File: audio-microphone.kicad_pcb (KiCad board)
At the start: 2 copper layers, 20 x 20 mm, 9 parts, among them J1 JST_SH_1x4_BM04B-SRSS-TB-LF-SN

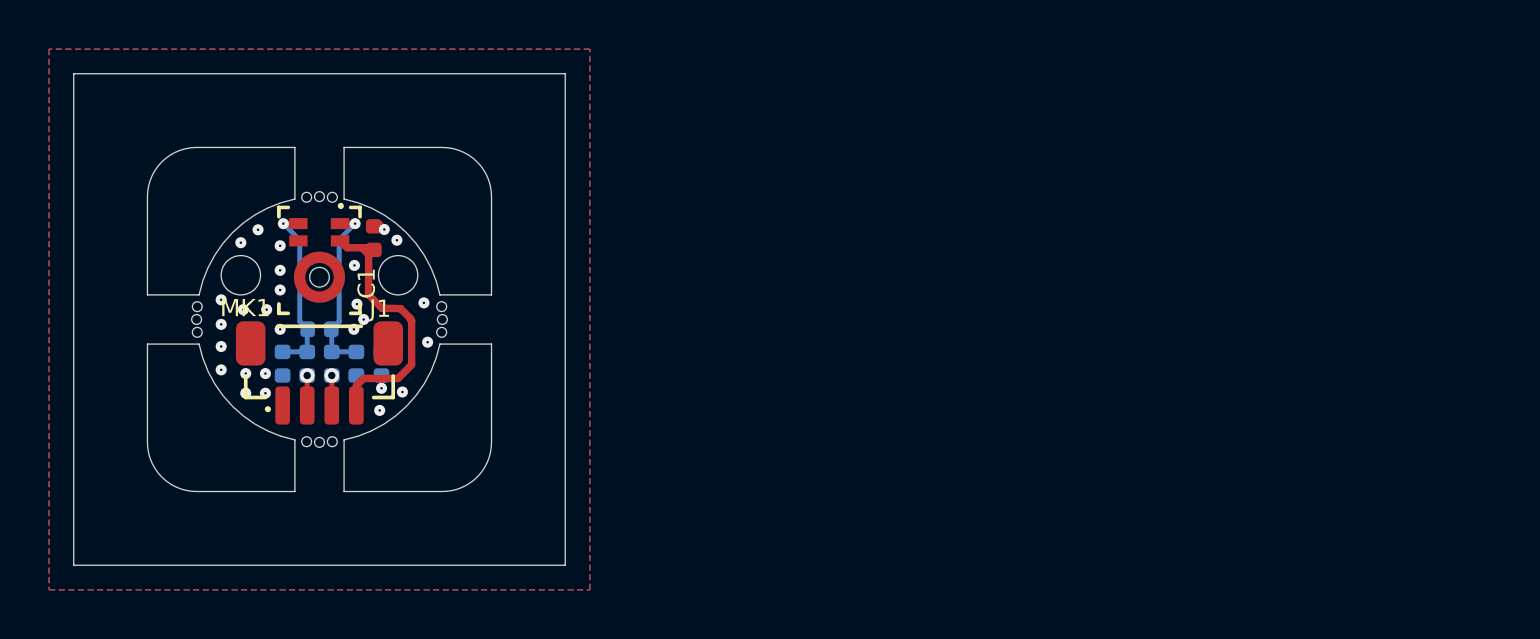
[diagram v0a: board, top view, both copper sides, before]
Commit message: [#71550] Start placement
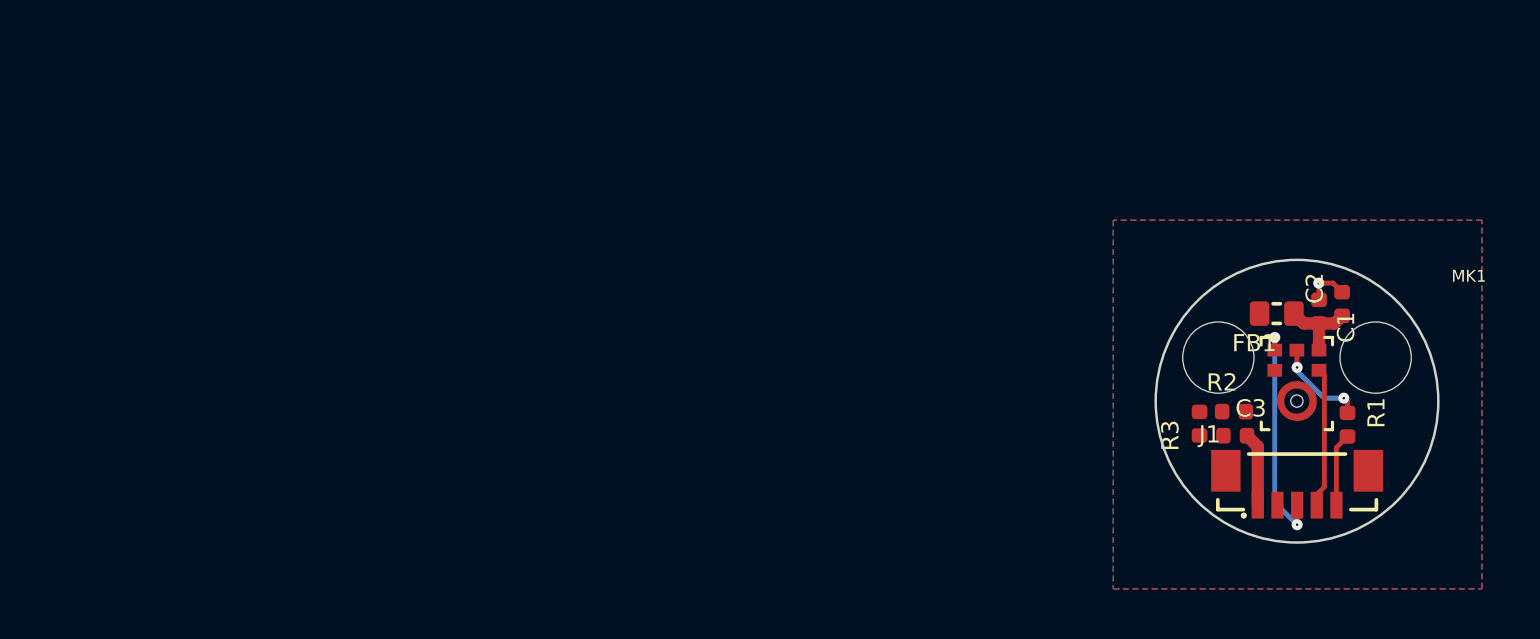
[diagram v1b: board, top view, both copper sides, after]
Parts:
- removed C4: C_100p_0402, antmicro-footprints:C_0402_1005Metric
- removed C5: C_100n_16V_X7R_0402, antmicro-footprints:C_0402_1005Metric
- added FB1: FB_600Z_0.5A_Murata-BLM18AG_0603, antmicro-footprints:FB_0603_1608Metric, F.Cu at (239.2, 143.4)
- added R3: R_0R_0402, antmicro-footprints:R_0402_1005Metric, F.Cu at (236.0, 147.8)
- C1: value C_100n_16V_X7R_0402 -> C_220p_0402
- C2: value C_100p_0402 -> C_100n_0402; moved to F.Cu
- C3: value C_100p_0402 -> C_1u_0402; moved to F.Cu
- J1: value JST_SH_1x4_BM04B-SRSS-TB-LF-SN -> JST_SH_1x5_BM05B-SURS-TB-LF-SN; footprint antmicro-footprints:Conn_JST_SH_1x4_BM04B-SRSS-TB-LF-SN -> antmicro-footprints:Conn_JST_SH_1x5_BM05B-SURS-TF-LF-SN
- MK1: value MK_IM73A135V01XTSA1 -> MK_SPH0645LM4H-B; footprint antmicro-footprints:MK_IM73A135V01XTSA1 -> antmicro-footprints:MK_SPH0645LM4H-B
- R1: value R_25k_0402 -> R_51R_0402; moved to F.Cu
- R2: value R_25k_0402 -> R_0R_0402; moved to F.Cu
- moved R1 41.4 mm to (242.0, 147.9), turned to -90 degrees
- moved C2 40.2 mm to (241.8, 143.0), turned to 90 degrees
- moved MK1 40.2 mm to (240.0, 146.9)
- moved J1 40.0 mm to (240.0, 150.2)
- moved C1 38.6 mm to (240.9, 143.3)
- moved R2 37.8 mm to (237.4, 147.3), turned to 0 degrees
- moved C3 37.5 mm to (237.5, 148.3)
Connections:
- C1 pad 2: +2V75 -> VDD
- C2 pad 1: Net-(MK1-OUTPUT+) -> VDD
- C3 pad 1: Net-(MK1-OUTPUT-) -> GND
- C3 pad 2: Net-(MK1-OUTPUT+) -> VCC
- J1 pad 1: GND -> VCC
- J1 pad 2: Net-(J1-Pad2) -> GND
- J1 pad 3: Net-(J1-Pad3) -> /WS
- J1 pad 4: +2V75 -> /BCLK
- MK1 pad 1: Net-(MK1-OUTPUT+) -> /WS
- MK1 pad 2: +2V75 -> /SELECT
- MK1 pad 3: Net-(MK1-OUTPUT-) -> GND
- MK1 pad 4: GND -> /BCLK
- MK1 pad 5: GND -> VDD
- R1 pad 1: Net-(J1-Pad3) -> Net-(MK1-DATA)
- R1 pad 2: Net-(MK1-OUTPUT+) -> /DATA
- R2 pad 1: Net-(MK1-OUTPUT-) -> /SELECT
- R2 pad 2: Net-(J1-Pad2) -> VDD
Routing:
- net +2V75: track 11.9 -> 0.00 mm, vias 1 -> 0
- net /WS: track 0.00 -> 9.31 mm, vias 0 -> 2
- net Net-(MK1-OUTPUT-): track 7.25 -> 0.00 mm, vias 1 -> 0
- net Net-(MK1-OUTPUT+): track 7.24 -> 0.00 mm, vias 1 -> 0
- net /BCLK: track 0.00 -> 5.71 mm
- net Net-(MK1-DATA): track 0.00 -> 3.88 mm, vias 0 -> 2
- net VDD: track 0.00 -> 3.34 mm
- net VCC: track 0.00 -> 3.01 mm
- net /DATA: track 0.00 -> 2.98 mm
- net GND: track 0.48 -> 1.79 mm, vias 26 -> 1
- net Net-(J1-Pad3): track 1.22 -> 0.00 mm, vias 1 -> 0
- net Net-(J1-Pad2): track 1.22 -> 0.00 mm, vias 1 -> 0
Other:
- board size 20 x 20 mm -> 11.5 x 11.5 mm
- board text removed: "Rev.${REVISION} Microphone"
- board text removed: "SHA ########"
